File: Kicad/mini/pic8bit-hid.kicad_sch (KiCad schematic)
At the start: 43 parts, among them K301 HARWIN-254-F-1X08-VERTICAL, K302 HARWIN-254-F-1X06-VERTICAL, P301 10k, P302 10k, U301 CAT4002A, U302 MCP2221A

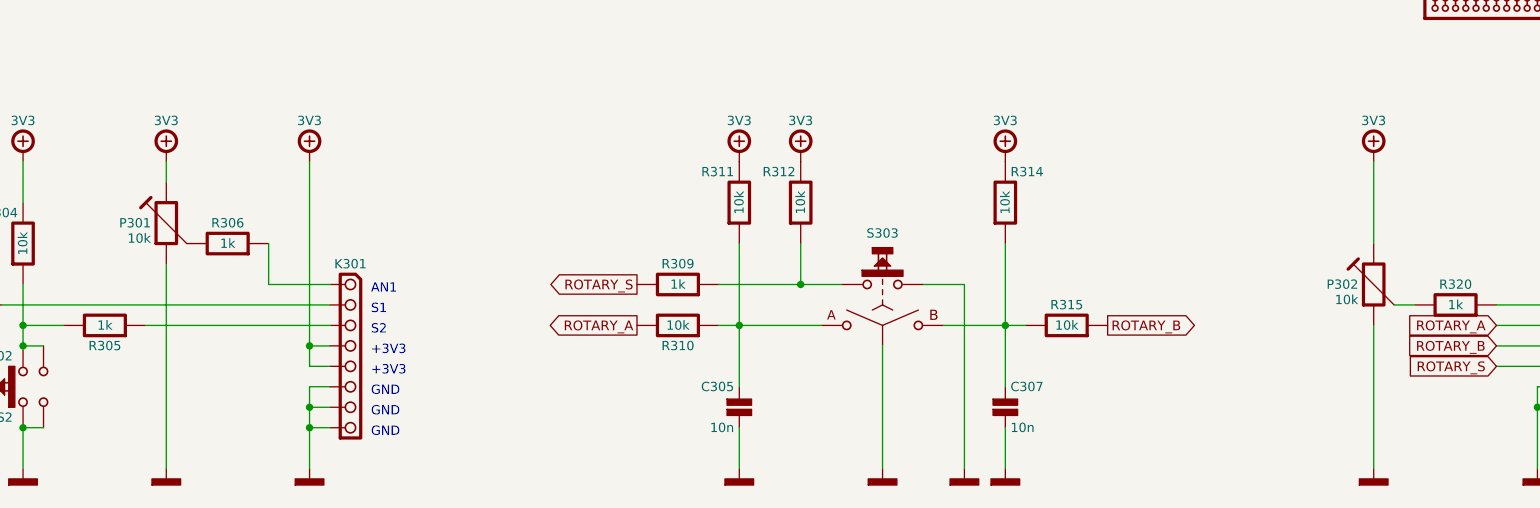
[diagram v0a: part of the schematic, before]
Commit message: Update Mini Kicad 8
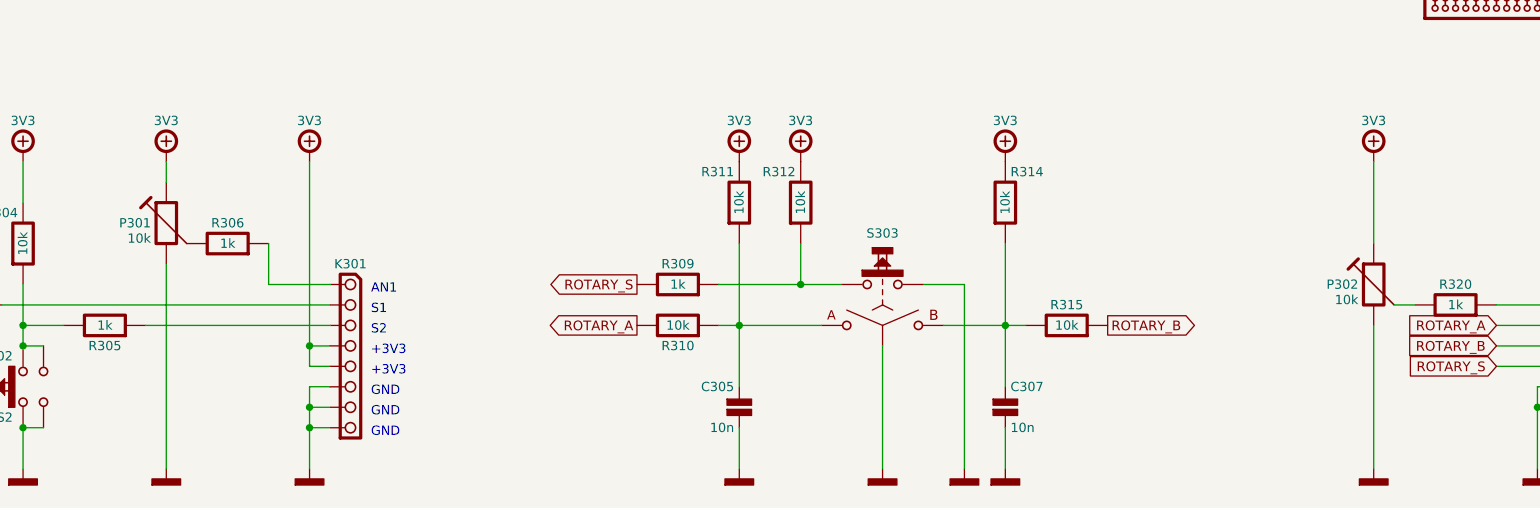
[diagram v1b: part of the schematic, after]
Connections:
- net +3V3 renamed POWER-+3V3
- net +5V renamed POWER-+5V
- net GND renamed POWER-GND
